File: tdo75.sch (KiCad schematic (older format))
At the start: 26 parts, among them SW1 SW_Push, U1 ATmega32U4-AU, Y1 16MHz

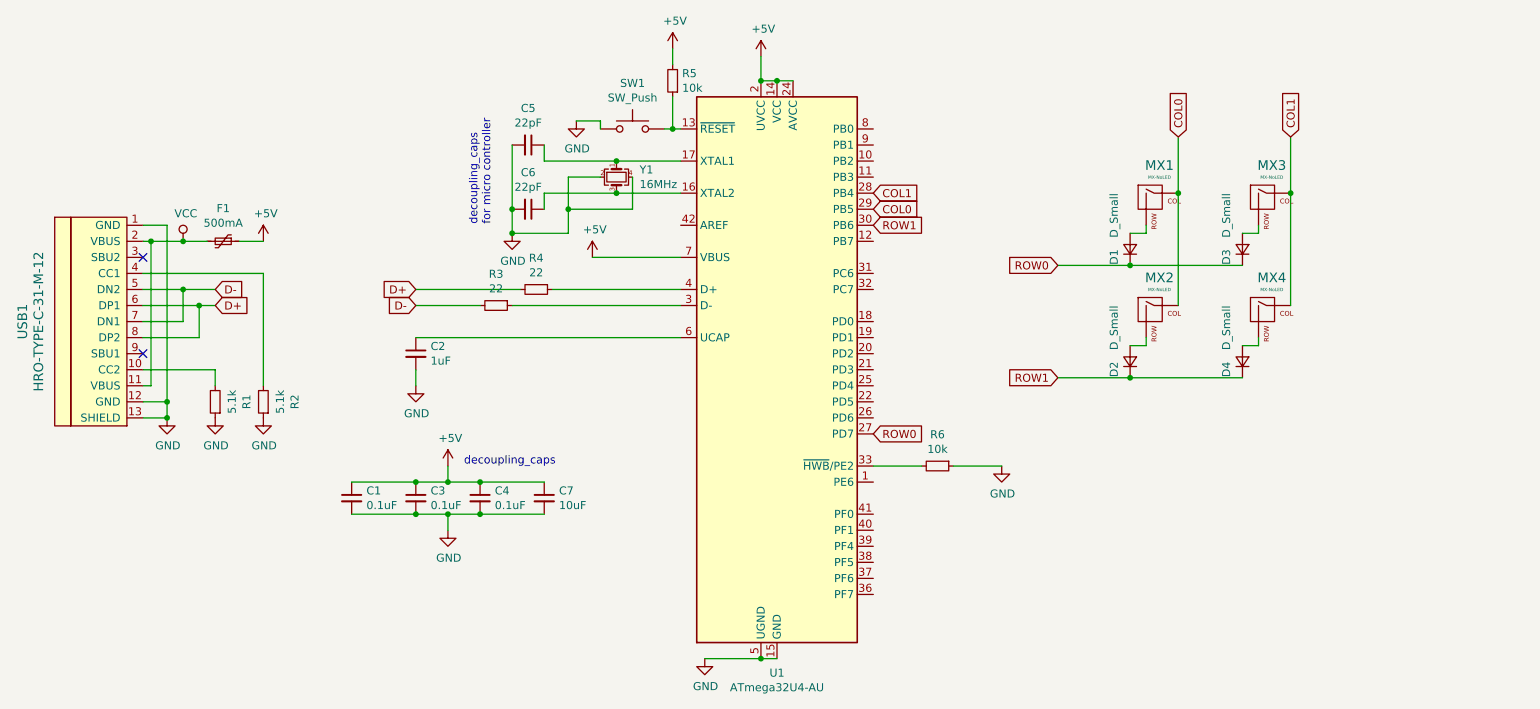
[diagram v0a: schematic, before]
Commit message: heirarchical keyboard matrix
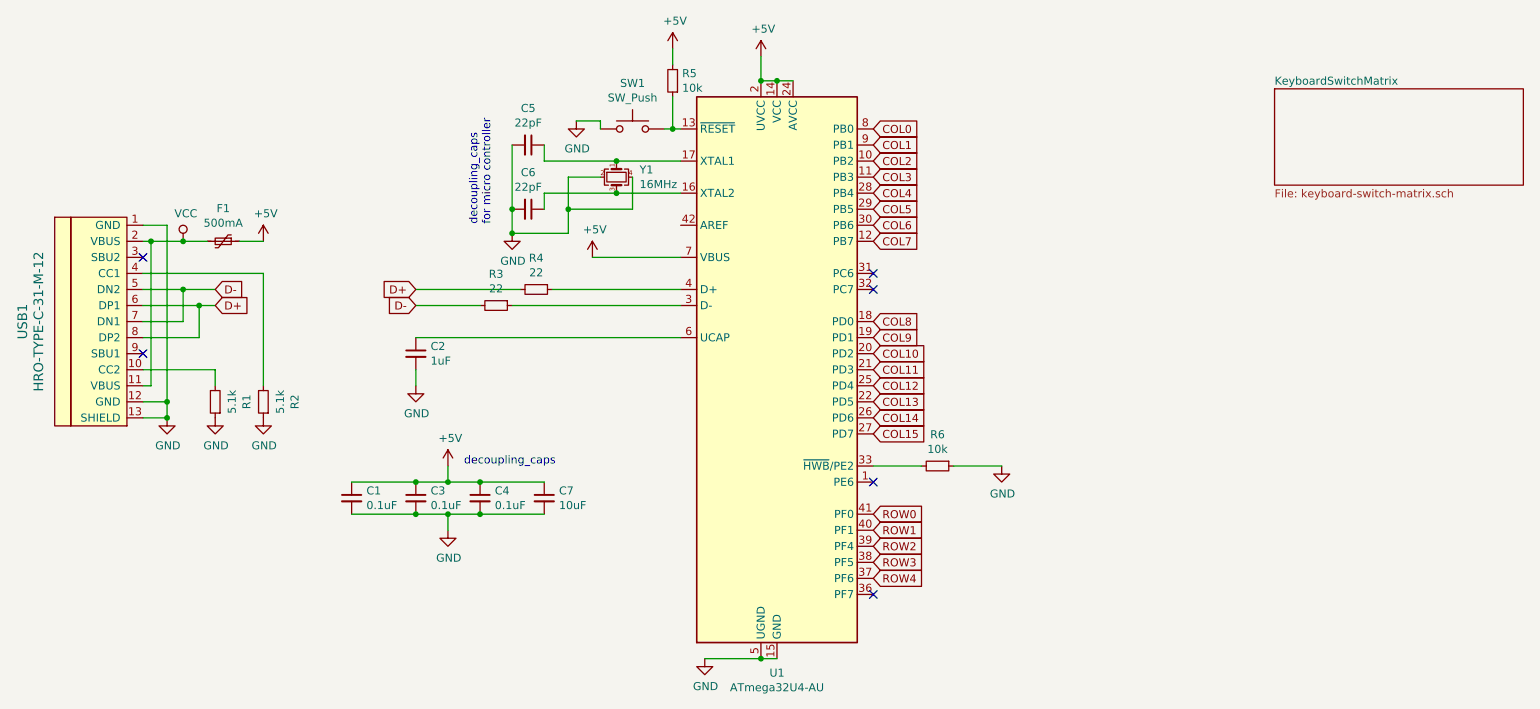
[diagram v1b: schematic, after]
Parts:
- removed D1, D2, D3, D4: D_Small, Diode_SMD:D_SOD-123, symbol Device:D_Small
- removed MX1, MX2, MX3, MX4: MX-NoLED, MX_Only:MXOnly-1U-NoLED, symbol MX_Alps_Hybrid:MX-NoLED
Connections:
- net COL0: now also U1.8 (PB0); no longer U1.29 (PB5)
- net COL1: now also U1.9 (PB1); no longer U1.28 (PB4)
- net ROW0: now also U1.41 (PF0); no longer U1.27 (PD7)
- net ROW1: now also U1.40 (PF1); no longer U1.30 (PB6)
- net COL2: now reaches U1.10 (PB2)
- net COL3: now reaches U1.11 (PB3)
- net COL7: now reaches U1.12 (PB7)
- net COL8: now reaches U1.18 (PD0)
- net COL9: now reaches U1.19 (PD1)
- net COL10: now reaches U1.20 (PD2)
- net COL11: now reaches U1.21 (PD3)
- net COL13: now reaches U1.22 (PD5)
- net COL12: now reaches U1.25 (PD4)
- net COL14: now reaches U1.26 (PD6)
- net ROW4: now reaches U1.37 (PF6)
- net ROW3: now reaches U1.38 (PF5)
- net ROW2: now reaches U1.39 (PF4)
- new net COL15: U1.27 (PD7)
- new net COL4: U1.28 (PB4)
- new net COL5: U1.29 (PB5)
- new net COL6: U1.30 (PB6)
- no-connect marks 2 -> 6
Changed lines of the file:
@@
 $Descr A4 11693 8268
 encoding utf-8
-Sheet 1 1
+Sheet 1 2
 Title ""
 Date ""
@@
 NoConn ~ 1550 4100
 NoConn ~ 1550 3500
-$Comp
-L MX_Alps_Hybrid:MX-NoLED MX1
-U 1 1 5E7B02A9
-P 7850 3150
-F 0 "MX1" H 7883 3373 60  0000 C CNN
-F 1 "MX-NoLED" H 7883 3299 20  0000 C CNN
-F 2 "MX_Only:MXOnly-1U-NoLED" H 7225 3125 60  0001 C CNN
-F 3 "" H 7225 3125 60  0001 C CNN
-	1    7850 3150
-	1    0    0    -1
-$EndComp
-$Comp
-L MX_Alps_Hybrid:MX-NoLED MX2
-U 1 1 5E7B0859
-P 7850 3850
-F 0 "MX2" H 7883 4073 60  0000 C CNN
-F 1 "MX-NoLED" H 7883 3999 20  0000 C CNN
-F 2 "MX_Only:MXOnly-1U-NoLED" H 7225 3825 60  0001 C CNN
-F 3 "" H 7225 3825 60  0001 C CNN
-	1    7850 3850
-	1    0    0    -1
-$EndComp
-$Comp
-L MX_Alps_Hybrid:MX-NoLED MX4
-U 1 1 5E7B0B55
-P 8550 3850
-F 0 "MX4" H 8583 4073 60  0000 C CNN
-F 1 "MX-NoLED" H 8583 3999 20  0000 C CNN
-F 2 "MX_Only:MXOnly-1U-NoLED" H 7925 3825 60  0001 C CNN
-F 3 "" H 7925 3825 60  0001 C CNN
-	1    8550 3850
-	1    0    0    -1
-$EndComp
-$Comp
-L MX_Alps_Hybrid:MX-NoLED MX3
-U 1 1 5E7B0E66
-P 8550 3150
-F 0 "MX3" H 8583 3373 60  0000 C CNN
-F 1 "MX-NoLED" H 8583 3299 20  0000 C CNN
-F 2 "MX_Only:MXOnly-1U-NoLED" H 7925 3125 60  0001 C CNN
-F 3 "" H 7925 3125 60  0001 C CNN
-	1    8550 3150
-	1    0    0    -1
-$EndComp
-$Comp
-L Device:D_Small D1
-U 1 1 5E7B3897
-P 7700 3450
-F 0 "D1" H 7700 3550 50  0000 R CNN
-F 1 "D_Small" H 8050 3550 50  0000 R CNN
-F 2 "Diode_SMD:D_SOD-123" V 7700 3450 50  0001 C CNN
-F 3 "~" V 7700 3450 50  0001 C CNN
-	1    7700 3450
-	0    -1   -1   0
-$EndComp
-Wire Wire Line
-	7700 3350 7800 3350
-Wire Wire Line
-	7800 3350 7800 3300
-$Comp
-L Device:D_Small D2
-U 1 1 5E7B58A6
-P 7700 4150
-F 0 "D2" H 7700 4250 50  0000 R CNN
-F 1 "D_Small" H 8050 4250 50  0000 R CNN
-F 2 "Diode_SMD:D_SOD-123" V 7700 4150 50  0001 C CNN
-F 3 "~" V 7700 4150 50  0001 C CNN
-	1    7700 4150
-	0    -1   -1   0
-$EndComp
-$Comp
-L Device:D_Small D4
-U 1 1 5E7B5B76
-P 8400 4150
-F 0 "D4" H 8400 4250 50  0000 R CNN
-F 1 "D_Small" H 8750 4250 50  0000 R CNN
-F 2 "Diode_SMD:D_SOD-123" V 8400 4150 50  0001 C CNN
-F 3 "~" V 8400 4150 50  0001 C CNN
-	1    8400 4150
-	0    -1   -1   0
-$EndComp
-$Comp
-L Device:D_Small D3
-U 1 1 5E7B5E2E
-P 8400 3450
-F 0 "D3" H 8400 3550 50  0000 R CNN
-F 1 "D_Small" H 8750 3550 50  0000 R CNN
-F 2 "Diode_SMD:D_SOD-123" V 8400 3450 50  0001 C CNN
-F 3 "~" V 8400 3450 50  0001 C CNN
-	1    8400 3450
-	0    -1   -1   0
-$EndComp
-Wire Wire Line
-	7700 4050 7800 4050
-Wire Wire Line
-	7800 4050 7800 4000
-Wire Wire Line
-	8400 4050 8500 4050
-Wire Wire Line
-	8500 4050 8500 4000
-Wire Wire Line
-	8400 3350 8500 3350
-Wire Wire Line
-	8500 3350 8500 3300
-Wire Wire Line
-	8000 3800 8000 3100
-Wire Wire Line
-	8000 3100 8000 2750
-Connection ~ 8000 3100
-Wire Wire Line
-	8400 3550 7700 3550
-Wire Wire Line
-	7700 3550 7250 3550
-Connection ~ 7700 3550
-Wire Wire Line
-	8400 4250 7700 4250
-Wire Wire Line
-	7700 4250 7250 4250
-Connection ~ 7700 4250
-Wire Wire Line
-	8700 3800 8700 3100
-Wire Wire Line
-	8700 3100 8700 2750
-Connection ~ 8700 3100
-Text GLabel 8000 2750 1    50   Input ~ 0
+Text GLabel 6100 2800 2    50   Input ~ 0
+COL1
+Text GLabel 6100 2700 2    50   Input ~ 0
 COL0
-Text GLabel 8700 2750 1    50   Input ~ 0
-COL1
-Text GLabel 7250 4250 0    50   Input ~ 0
-ROW1
-Text GLabel 7250 3550 0    50   Input ~ 0
+Text GLabel 6100 5100 2    50   Input ~ 0
 ROW0
-Text GLabel 6100 3100 2    50   Input ~ 0
-COL1
-Text GLabel 6100 3200 2    50   Input ~ 0
-COL0
-Text GLabel 6100 4600 2    50   Input ~ 0
-ROW0
-Text GLabel 6100 3300 2    50   Input ~ 0
+Text GLabel 6100 5200 2    50   Input ~ 0
 ROW1
 Wire Wire Line
@@
 Wire Wire Line
 	2150 3400 2300 3400
+$Sheet
+S 8600 2450 1550 600
+U 5E80119E
+F0 "KeyboardSwitchMatrix" 50
+F1 "keyboard-switch-matrix.sch" 50
+$EndSheet
+Text GLabel 6100 2900 2    50   Input ~ 0
+COL2
+Text GLabel 6100 3000 2    50   Input ~ 0
+COL3
+Text GLabel 6100 3100 2    50   Input ~ 0
+COL4
+Text GLabel 6100 3200 2    50   Input ~ 0
+COL5
+Text GLabel 6100 3300 2    50   Input ~ 0
+COL6
+Text GLabel 6100 3400 2    50   Input ~ 0
+COL7
+Text GLabel 6100 3900 2    50   Input ~ 0
+COL8
+Text GLabel 6100 4000 2    50   Input ~ 0
+COL9
+Text GLabel 6100 4100 2    50   Input ~ 0
+COL10
+Text GLabel 6100 4200 2    50   Input ~ 0
+COL11
+Text GLabel 6100 4300 2    50   Input ~ 0
+COL12
+Text GLabel 6100 4400 2    50   Input ~ 0
+COL13
+Text GLabel 6100 4500 2    50   Input ~ 0
+COL14
+Text GLabel 6100 4600 2    50   Input ~ 0
+COL15
+Text GLabel 6100 5300 2    50   Input ~ 0
+ROW2
+Text GLabel 6100 5400 2    50   Input ~ 0
+ROW3
+Text GLabel 6100 5500 2    50   Input ~ 0
+ROW4
+NoConn ~ 6100 5600
+NoConn ~ 6100 4900
+NoConn ~ 6100 3600
+NoConn ~ 6100 3700
 $EndSCHEMATC
